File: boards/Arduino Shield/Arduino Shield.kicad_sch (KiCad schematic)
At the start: 6 parts, among them J1 Screw_Terminal_01x09, J2 Screw_Terminal_01x09, J3 Screw_Terminal_01x09, J4 Screw_Terminal_01x09, J5 Screw_Terminal_01x09, J6 Screw_Terminal_01x09

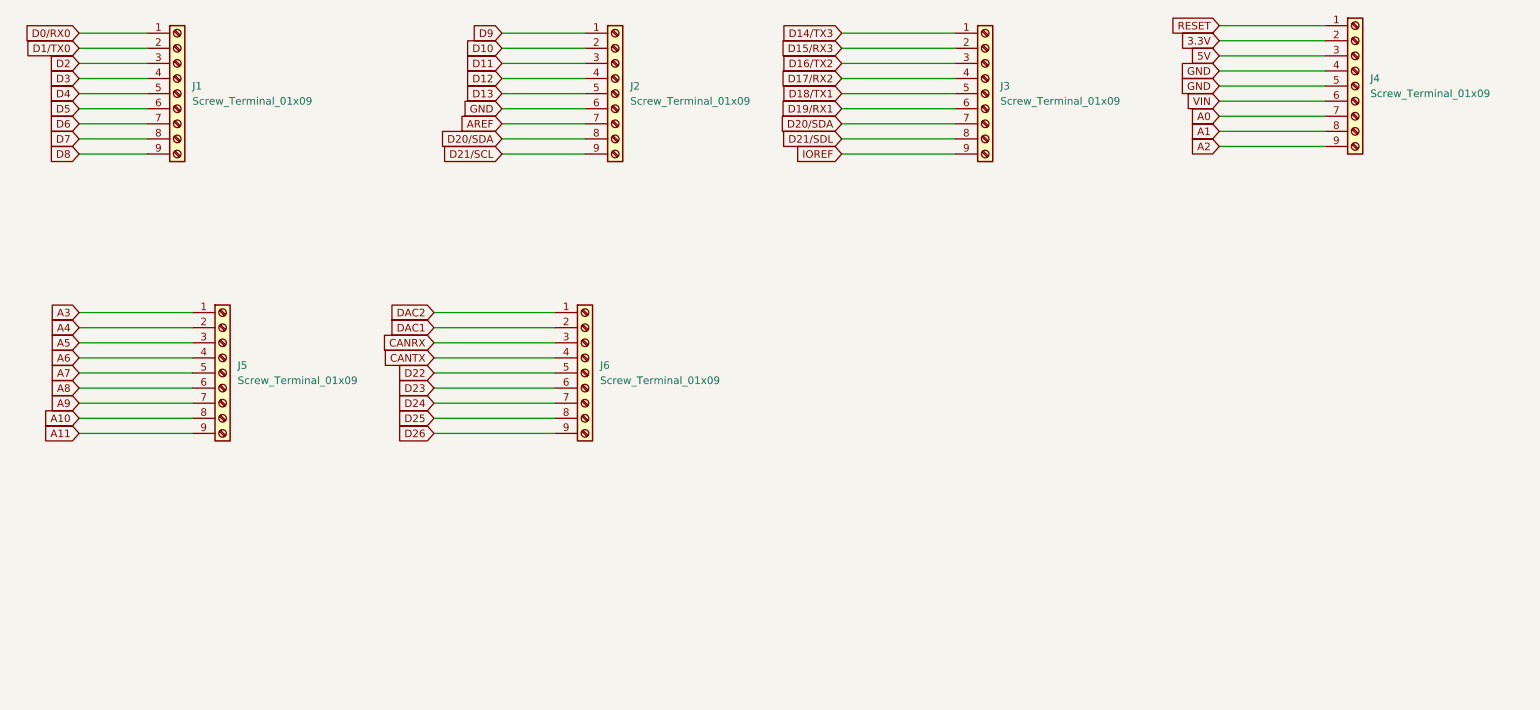
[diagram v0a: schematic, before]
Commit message: Shield Schematic
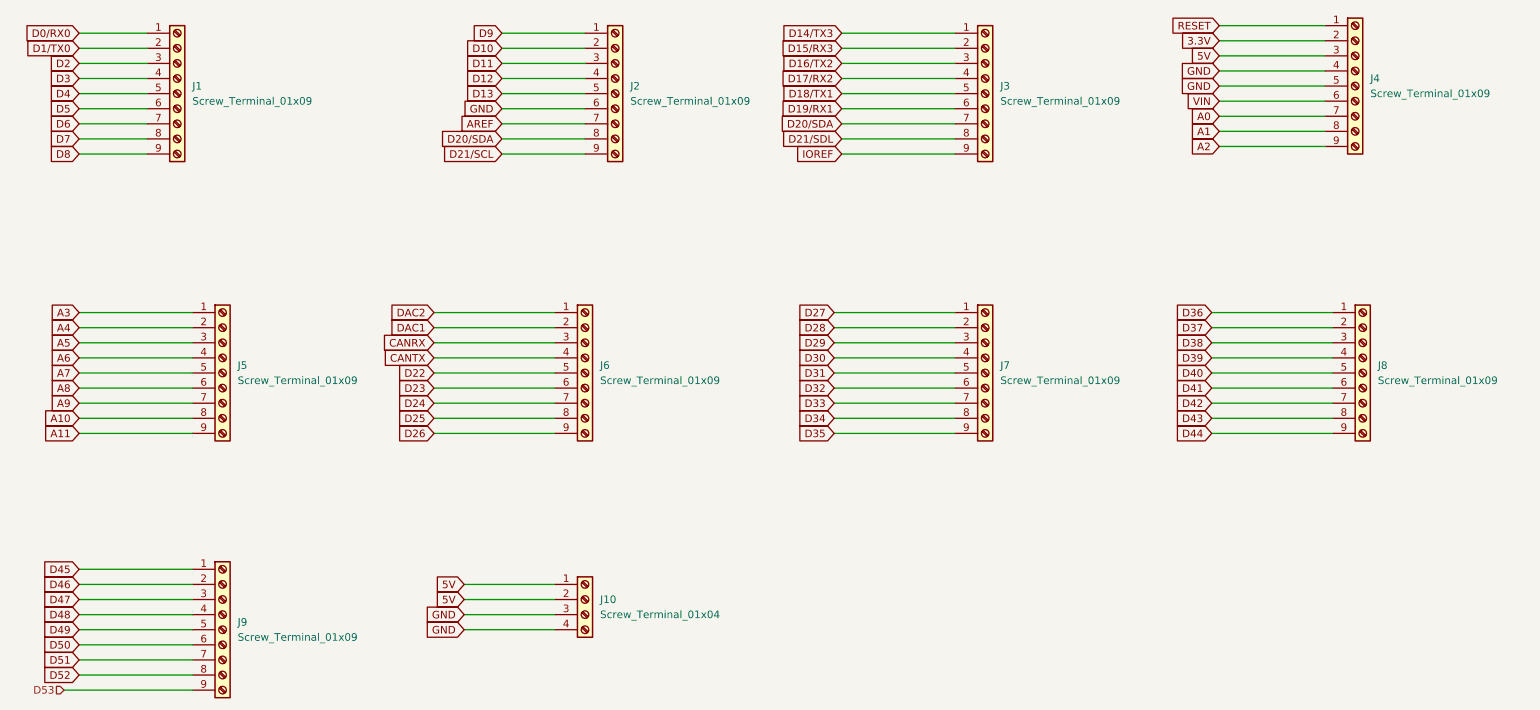
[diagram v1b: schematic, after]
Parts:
- added J10: Screw_Terminal_01x04, symbol Connector:Screw_Terminal_01x04
- added J7, J8, J9: Screw_Terminal_01x09, symbol Connector:Screw_Terminal_01x09
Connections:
- net 5V: now also J10.1 (Pin_1), J10.2 (Pin_2)
- net GND: now also J10.3 (Pin_3), J10.4 (Pin_4)
- new net D27: J7.1 (Pin_1)
- new net D28: J7.2 (Pin_2)
- new net D29: J7.3 (Pin_3)
- new net D30: J7.4 (Pin_4)
- new net D31: J7.5 (Pin_5)
- new net D32: J7.6 (Pin_6)
- new net D33: J7.7 (Pin_7)
- new net D34: J7.8 (Pin_8)
- new net D35: J7.9 (Pin_9)
- new net D36: J8.1 (Pin_1)
- new net D37: J8.2 (Pin_2)
- new net D38: J8.3 (Pin_3)
- new net D39: J8.4 (Pin_4)
- new net D40: J8.5 (Pin_5)
- new net D41: J8.6 (Pin_6)
- new net D42: J8.7 (Pin_7)
- new net D43: J8.8 (Pin_8)
- new net D44: J8.9 (Pin_9)
- new net D45: J9.1 (Pin_1)
- new net D46: J9.2 (Pin_2)
- new net D47: J9.3 (Pin_3)
- new net D48: J9.4 (Pin_4)
- new net D49: J9.5 (Pin_5)
- new net D50: J9.6 (Pin_6)
- new net D51: J9.7 (Pin_7)
- new net D52: J9.8 (Pin_8)
- new net D53: J9.9 (Pin_9)
